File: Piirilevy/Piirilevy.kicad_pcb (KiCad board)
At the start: 2 copper layers, 21 parts, among them J1 Conn_01x02, J2 Conn_01x02_Pin, J3 Conn_01x19_Socket, J4 Conn_02x03_Odd_Even, J5 Conn_01x19_Socket, J6 Conn_01x03_Socket, U1 ATmega8535-16P, U3 LM3940IMP-3.3, U6 L7805

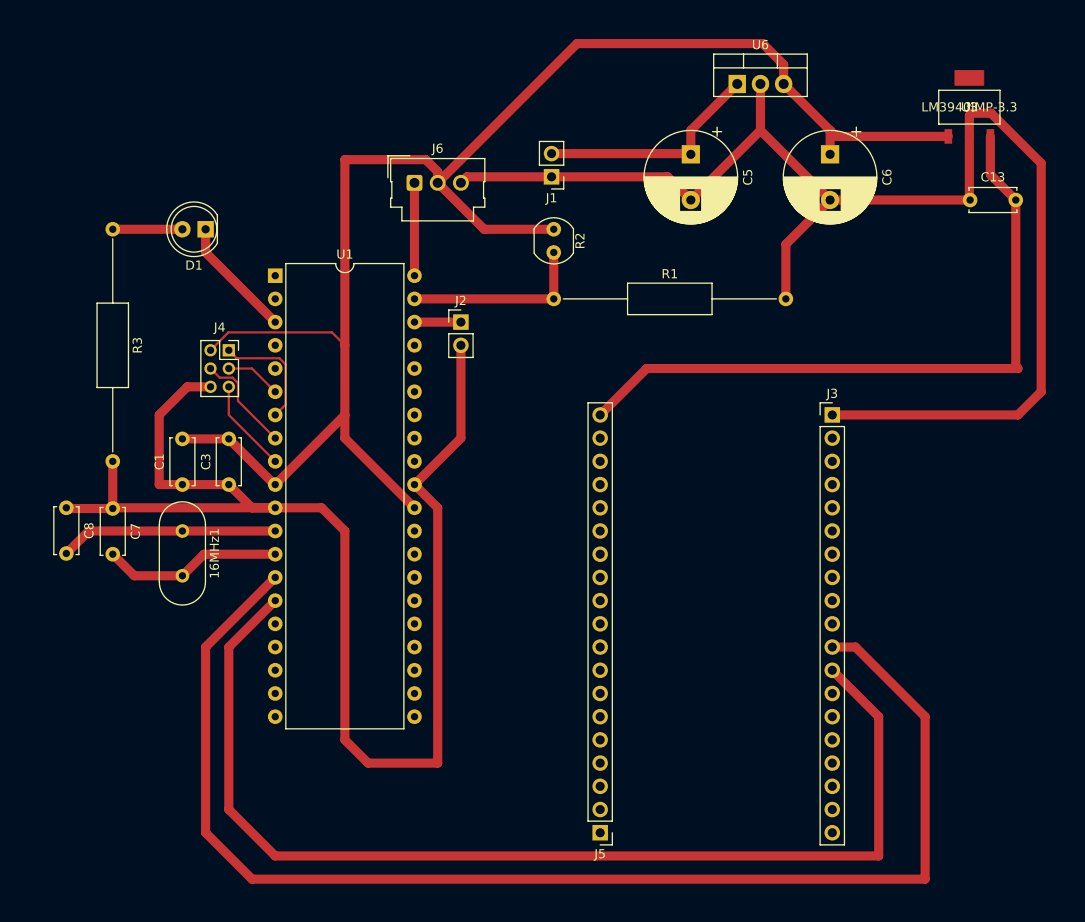
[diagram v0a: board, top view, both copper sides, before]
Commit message: Piirilevy suunnitelu valmis
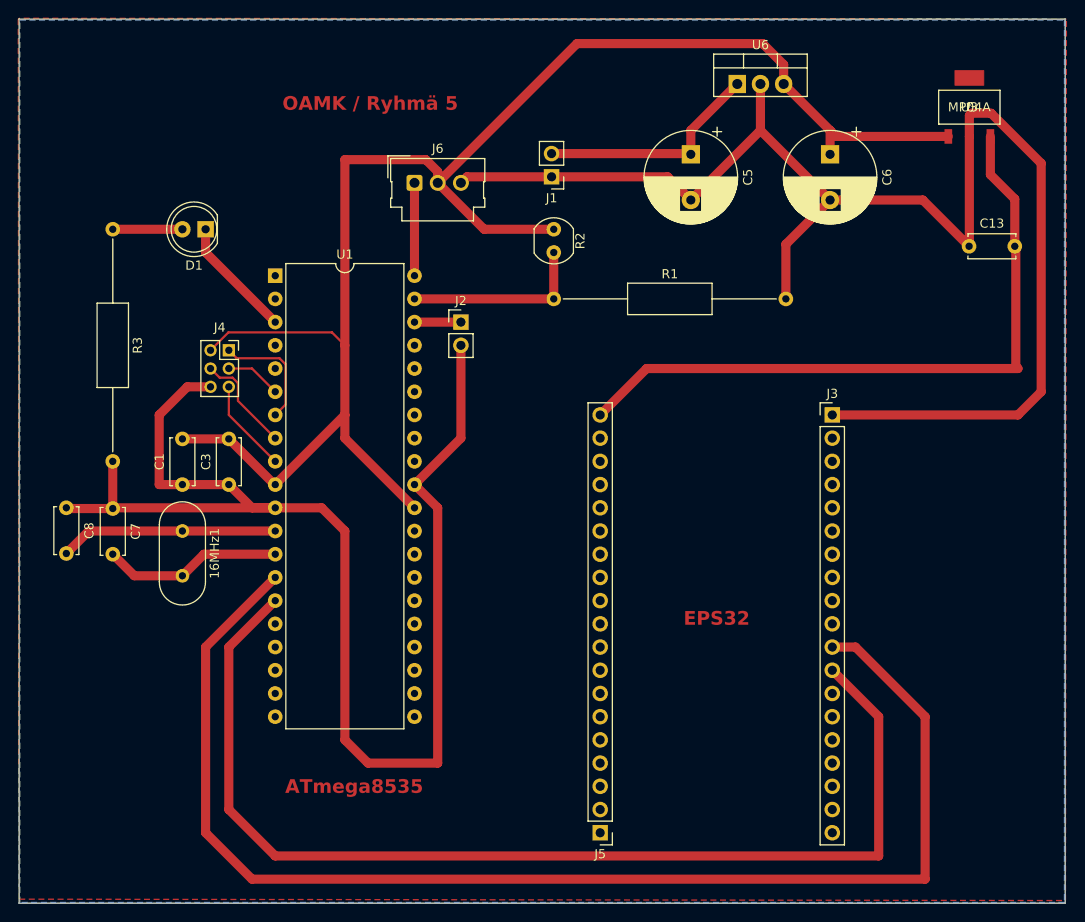
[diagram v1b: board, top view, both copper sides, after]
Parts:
- U3: value LM3940IMP-3.3 -> MP04A; footprint Oma:LM3940IMP-3.3 -> footprints:LM3940IMP-3.3
- moved C13 5.06 mm to (147.1, 42.5)
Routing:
- net GND: track 297.7 -> 304.7 mm
- net Net-(J4-Pin_5): track 10.8 -> 10.3 mm
- added copper zone on B.Cu, net GND
- added copper zone on F.Cu, net GND
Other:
- board outline added: 114.5 x 96.8 mm
- board text added: "ATmega8535"
- board text added: "EPS32"
- board text added: "OAMK / Ryhmä 5"
